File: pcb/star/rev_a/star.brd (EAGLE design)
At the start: 47 x 40 mm, 42 parts, among them J2 TC2030-JLINK-NL, J3 MICRO_USB_B_HIROSE_ZX62-B-5PA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, J4 TC2030-JLINK-NL, U2 LTC4065, U3 TRIPOINT, U4 TPS715AXX, U5 NRF51822QF, X1 EPSON-FA-128

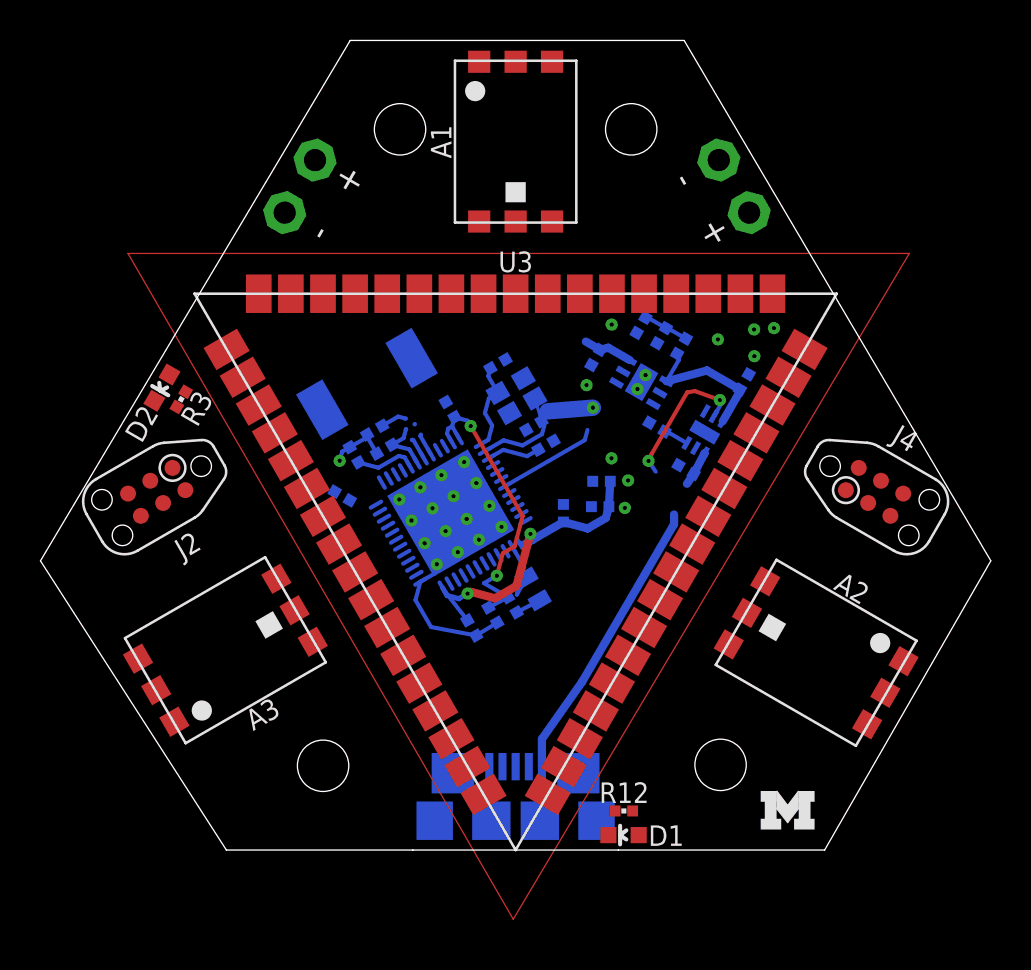
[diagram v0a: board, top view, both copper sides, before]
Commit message: fixed up dimensions
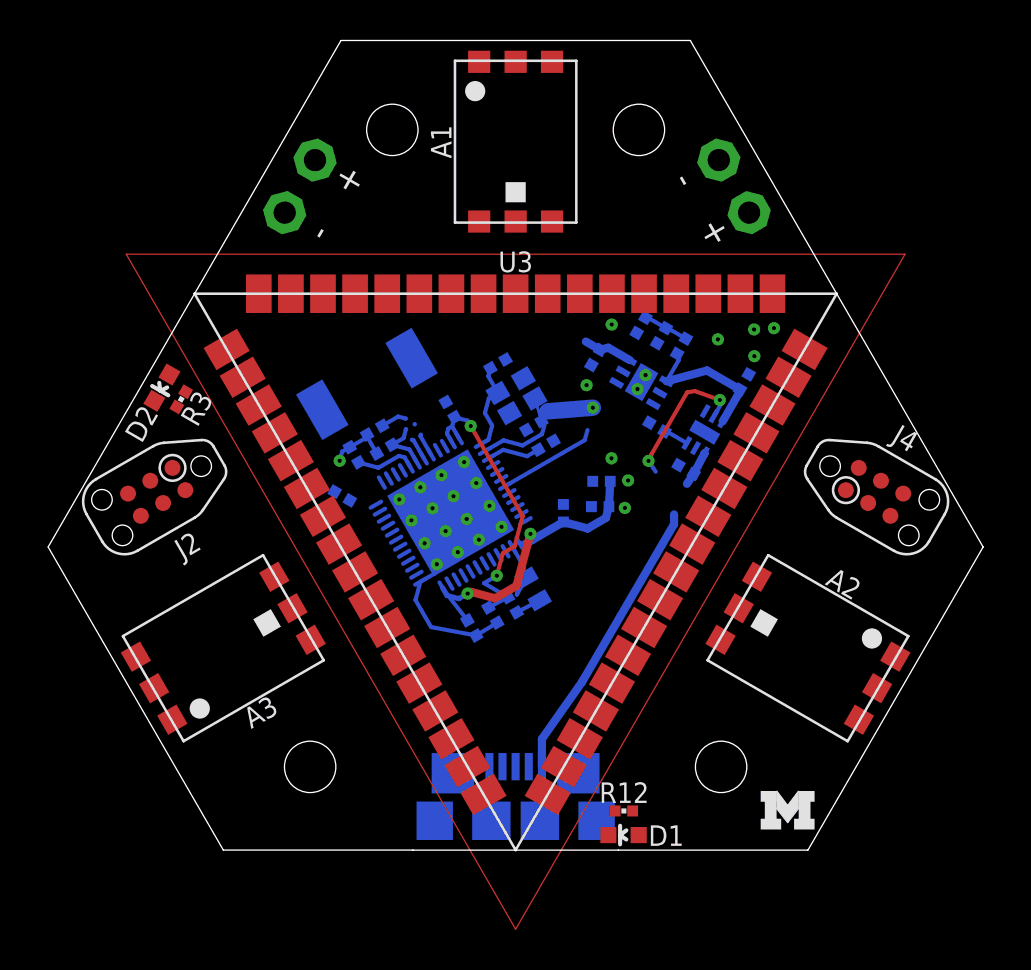
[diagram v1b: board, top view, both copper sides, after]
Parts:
- moved A2 0.47 mm to (14.5, -8.36)
- moved A3 0.14 mm to (-14.5, -8.36)
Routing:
- net GND: track 127.5 -> 128.1 mm
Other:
- board size 47 x 40 mm -> 46.2 x 40 mm
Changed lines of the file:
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@@
 <board>
 <plain>
-<wire x1="-8.178803125" y1="21.693628125" x2="8.331196875" y2="21.693628125" width="0" layer="20"/>
-<wire x1="8.331196875" y1="21.693628125" x2="23.494996875" y2="-4.03656875" width="0" layer="20"/>
-<wire x1="23.494996875" y1="-4.03656875" x2="15.27718125" y2="-18.33676875" width="0" layer="20"/>
-<wire x1="-14.301196875" y1="-18.33676875" x2="-23.495003125" y2="-4.036575" width="0" layer="20"/>
-<wire x1="-23.495003125" y1="-4.036575" x2="-8.178803125" y2="21.693628125" width="0" layer="20"/>
-<wire x1="-14.301196875" y1="-18.33676875" x2="-5.080003125" y2="-18.33676875" width="0" layer="20"/>
-<wire x1="5.08" y1="-18.33676875" x2="15.27718125" y2="-18.33676875" width="0" layer="20"/>
-<hole x="10.13289375" y="-14.124225" drill="2.54"/>
-<hole x="-9.52028125" y="-14.169271875" drill="2.54"/>
-<hole x="-5.715003125" y="17.299428125" drill="2.54"/>
-<hole x="5.714996875" y="17.29943125" drill="2.54"/>
+<wire x1="-8.636" y1="21.6916" x2="8.636" y2="21.6916" width="0" layer="20"/>
+<wire x1="8.636" y1="21.6916" x2="23.114" y2="-3.3528" width="0" layer="20"/>
+<wire x1="23.114" y1="-3.3528" x2="14.4526" y2="-18.3388" width="0" layer="20"/>
+<wire x1="-14.4526" y1="-18.33676875" x2="-23.114" y2="-3.3528" width="0" layer="20"/>
+<wire x1="-23.114" y1="-3.3528" x2="-8.636" y2="21.6916" width="0" layer="20"/>
+<wire x1="-14.4526" y1="-18.33676875" x2="-5.08" y2="-18.33676875" width="0" layer="20"/>
+<wire x1="5.08" y1="-18.3388" x2="14.4526" y2="-18.3388" width="0" layer="20"/>
+<hole x="10.16" y="-14.224" drill="2.54"/>
+<hole x="-10.16" y="-14.224" drill="2.54"/>
+<hole x="-6.096" y="17.272" drill="2.54"/>
+<hole x="6.096" y="17.272" drill="2.54"/>
 </plain>
 <attributes>
@@
 </autorouter>
 <elements>
-<element name="A1" library="chips" package="TAIYO-YUDEN-AH086M" value="TAIYO-YUDEN-AH086M" x="0" y="16.68983125" smashed="yes">
-<attribute name="DIGIKEY" value="587-2204-1-ND" x="16.509996875" y="11.609828125" size="1.778" layer="27" display="off"/>
-<attribute name="NAME" x="-3.17323125" y="16.6878" size="1.016" layer="25" font="vector" ratio="12" rot="R90" align="bottom-center"/>
-</element>
-<element name="A2" library="chips" package="TAIYO-YUDEN-AH086M" value="TAIYO-YUDEN-AH086M" x="14.858996875" y="-8.58316875" smashed="yes" rot="R240">
-<attribute name="DIGIKEY" value="587-2204-1-ND" x="-0.970409375" y="-25.840509375" size="1.778" layer="27" rot="R240" display="off"/>
-<attribute name="NAME" x="16.39176875" y="-5.829878125" size="1.016" layer="25" font="vector" ratio="12" rot="R330" align="bottom-center"/>
-</element>
-<element name="A3" library="chips" package="TAIYO-YUDEN-AH086M" value="TAIYO-YUDEN-AH086M" x="-14.351003125" y="-8.45616875" smashed="yes" rot="R120">
-<attribute name="DIGIKEY" value="587-2204-1-ND" x="-8.307925" y="14.09690625" size="1.778" layer="27" rot="R120" display="off"/>
-<attribute name="NAME" x="-12.767434375" y="-11.162728125" size="1.016" layer="25" font="vector" ratio="12" rot="R210" align="bottom-center"/>
+<element name="A1" library="chips" package="TAIYO-YUDEN-AH086M" value="TAIYO-YUDEN-AH086M" x="0" y="16.6878" smashed="yes">
+<attribute name="DIGIKEY" value="587-2204-1-ND" x="16.509996875" y="11.607796875" size="1.778" layer="27" display="off"/>
+<attribute name="NAME" x="-3.17323125" y="16.68576875" size="1.016" layer="25" font="vector" ratio="12" rot="R90" align="bottom-center"/>
+</element>
+<element name="A2" library="chips" package="TAIYO-YUDEN-AH086M" value="TAIYO-YUDEN-AH086M" x="14.4526" y="-8.3566" smashed="yes" rot="R240">
+<attribute name="DIGIKEY" value="587-2204-1-ND" x="-1.37680625" y="-25.613940625" size="1.778" layer="27" rot="R240" display="off"/>
+<attribute name="NAME" x="15.985371875" y="-5.603309375" size="1.016" layer="25" font="vector" ratio="12" rot="R330" align="bottom-center"/>
+</element>
+<element name="A3" library="chips" package="TAIYO-YUDEN-AH086M" value="TAIYO-YUDEN-AH086M" x="-14.4526" y="-8.3566" smashed="yes" rot="R120">
+<attribute name="DIGIKEY" value="587-2204-1-ND" x="-8.409521875" y="14.196475" size="1.778" layer="27" rot="R120" display="off"/>
+<attribute name="NAME" x="-12.86903125" y="-11.063159375" size="1.016" layer="25" font="vector" ratio="12" rot="R210" align="bottom-center"/>
 </element>
 <element name="X1" library="crystals" package="FA-128" value="EPSON-FA-128" x="0.040640625" y="4.12666875" smashed="yes" rot="MR150">
@@
 <attribute name="VALUE" x="-17.914746875" y="5.944984375" size="0.4064" layer="27" rot="R240"/>
 </element>
-<element name="J3" library="connector" package="USB_MICRO_B-HIROSE-ZX62-B-5PA(11)" value="MICRO_USB_B_HIROSE_ZX62-B-5PA(11)" x="0" y="-18.33676875" rot="MR0">
-<attribute name="MOUSER" value="798-ZX62-B-5PA11" x="0" y="-18.33676875" size="1.778" layer="28" rot="MR0" display="off"/>
-<attribute name="NEWARK" value="86P8793" x="0" y="-18.33676875" size="1.778" layer="28" rot="MR0" display="off"/>
-<attribute name="DIGIKEY" value="H11634CT-ND" x="0" y="-18.33676875" size="1.778" layer="28" rot="MR0" display="off"/>
+<element name="J3" library="connector" package="USB_MICRO_B-HIROSE-ZX62-B-5PA(11)" value="MICRO_USB_B_HIROSE_ZX62-B-5PA(11)" x="0" y="-18.3388" rot="MR0">
+<attribute name="MOUSER" value="798-ZX62-B-5PA11" x="0" y="-18.3388" size="1.778" layer="28" rot="MR0" display="off"/>
+<attribute name="NEWARK" value="86P8793" x="0" y="-18.3388" size="1.778" layer="28" rot="MR0" display="off"/>
+<attribute name="DIGIKEY" value="H11634CT-ND" x="0" y="-18.3388" size="1.778" layer="28" rot="MR0" display="off"/>
 </element>
 <element name="U3" library="tripoint" package="TRIPOINT" value="TRIPOINT" x="0" y="0"/>
@@
 <wire x1="3.819071875" y1="3.535628125" x2="1.5793875" y2="3.35624375" width="0.8128" layer="16"/>
 <contactref element="J3" pad="5"/>
-<wire x1="-19.167390625" y1="11.162290625" x2="-0.117390625" y2="-21.756109375" width="0" layer="1"/>
-<wire x1="-0.117390625" y1="-21.756109375" x2="19.466009375" y2="11.162290625" width="0" layer="1"/>
-<wire x1="19.466009375" y1="11.162290625" x2="-19.167390625" y2="11.162290625" width="0" layer="1"/>
+<wire x1="-19.2532" y1="11.1252" x2="0" y2="-22.2504" width="0" layer="1"/>
+<wire x1="0" y1="-22.2504" x2="19.2532" y2="11.1252" width="0" layer="1"/>
+<wire x1="19.2532" y1="11.1252" x2="-19.2532" y2="11.1252" width="0" layer="1"/>
 <contactref element="U$4" pad="N"/>
 <contactref element="U$3" pad="N"/>
@@
 <wire x1="-6.862209375" y1="1.268534375" x2="-4.9900625" y2="2.718665625" width="0" layer="19" extent="16-16"/>
 <wire x1="-8.19645625" y1="-1.045490625" x2="-8.70006875" y2="0.911309375" width="0" layer="19" extent="16-16"/>
-<wire x1="-1.3" y1="-14.21176875" x2="-1.952625" y2="-7.729175" width="0" layer="19" extent="16-16"/>
-<wire x1="19.466009375" y1="11.162290625" x2="12.7727375" y2="7.466778125" width="0" layer="19" extent="1-1"/>
-<wire x1="-11.418" y1="13.178959375" x2="-19.167390625" y2="11.162290625" width="0" layer="19" extent="1-1"/>
+<wire x1="-1.3" y1="-14.2138" x2="-1.952625" y2="-7.729175" width="0" layer="19" extent="16-16"/>
+<wire x1="19.2532" y1="11.1252" x2="12.7727375" y2="7.466778125" width="0" layer="19" extent="1-1"/>
+<wire x1="-11.418" y1="13.178959375" x2="-19.2532" y2="11.1252" width="0" layer="19" extent="1-1"/>
 <wire x1="18.52935625" y1="-1.811671875" x2="11.525375" y2="5.18295625" width="0" layer="19" extent="1-16"/>
 <wire x1="-19.16435625" y1="-0.71181875" x2="-8.70006875" y2="0.911309375" width="0" layer="19" extent="1-1"/>
@@
 <wire x1="8.80435" y1="0.26226875" x2="8.4719375" y2="-0.227078125" width="0.4064" layer="16"/>
 <contactref element="J3" pad="1"/>
-<wire x1="1.3" y1="-14.21176875" x2="1.3" y2="-12.84571875" width="0.4064" layer="16"/>
+<wire x1="1.3" y1="-14.2138" x2="1.3" y2="-12.84571875" width="0.4064" layer="16"/>
 <wire x1="1.3" y1="-12.84571875" x2="3.286209375" y2="-10.021309375" width="0.4064" layer="16"/>
 <wire x1="3.286209375" y1="-10.021309375" x2="7.832809375" y2="-2.223509375" width="0.4064" layer="16"/>
 <wire x1="7.832809375" y1="-2.223509375" x2="7.832809375" y2="-1.743046875" width="0.4064" layer="16"/>
-<wire x1="1.3" y1="-14.21176875" x2="4.918759375" y2="-16.402353125" width="0" layer="19" extent="1-16"/>
+<wire x1="1.3" y1="-14.2138" x2="4.918759375" y2="-16.402353125" width="0" layer="19" extent="1-16"/>
 <wire x1="8.4719375" y1="-0.227078125" x2="7.832809375" y2="-1.743046875" width="0" layer="19" extent="16-16"/>
 </signal>

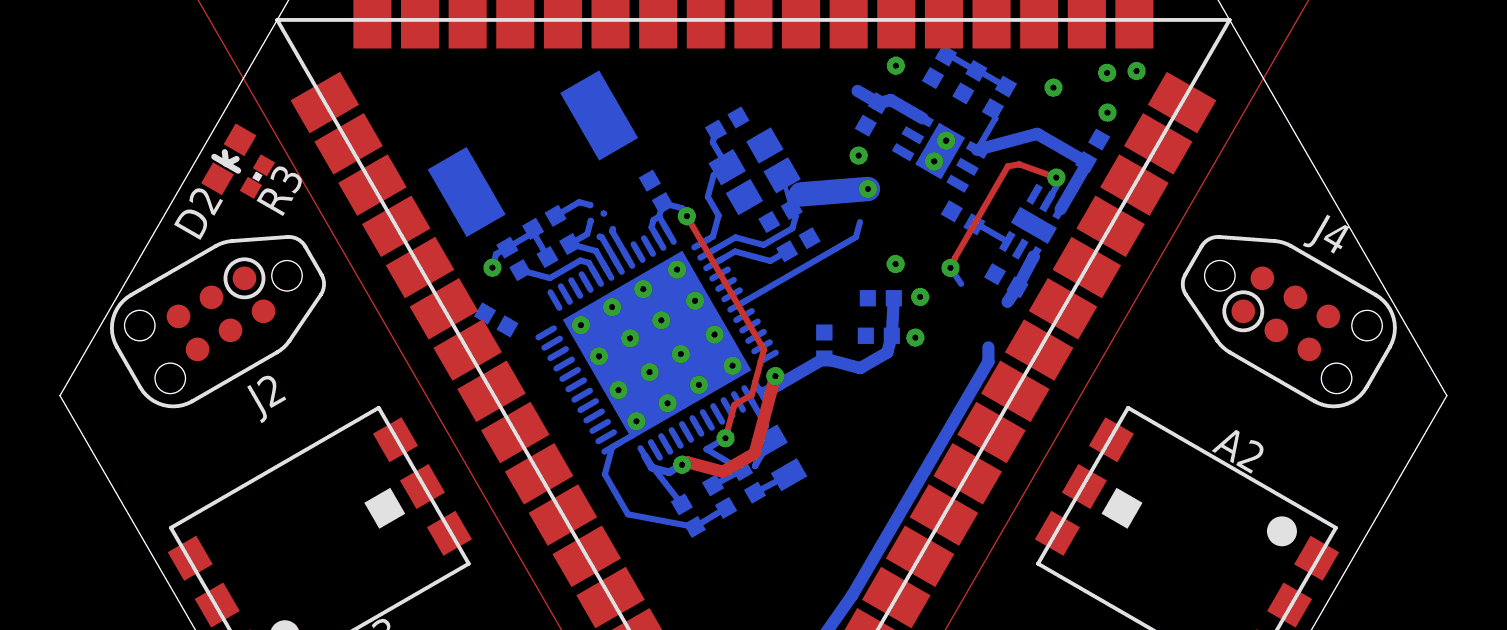
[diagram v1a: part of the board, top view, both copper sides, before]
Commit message: much farther on anchor
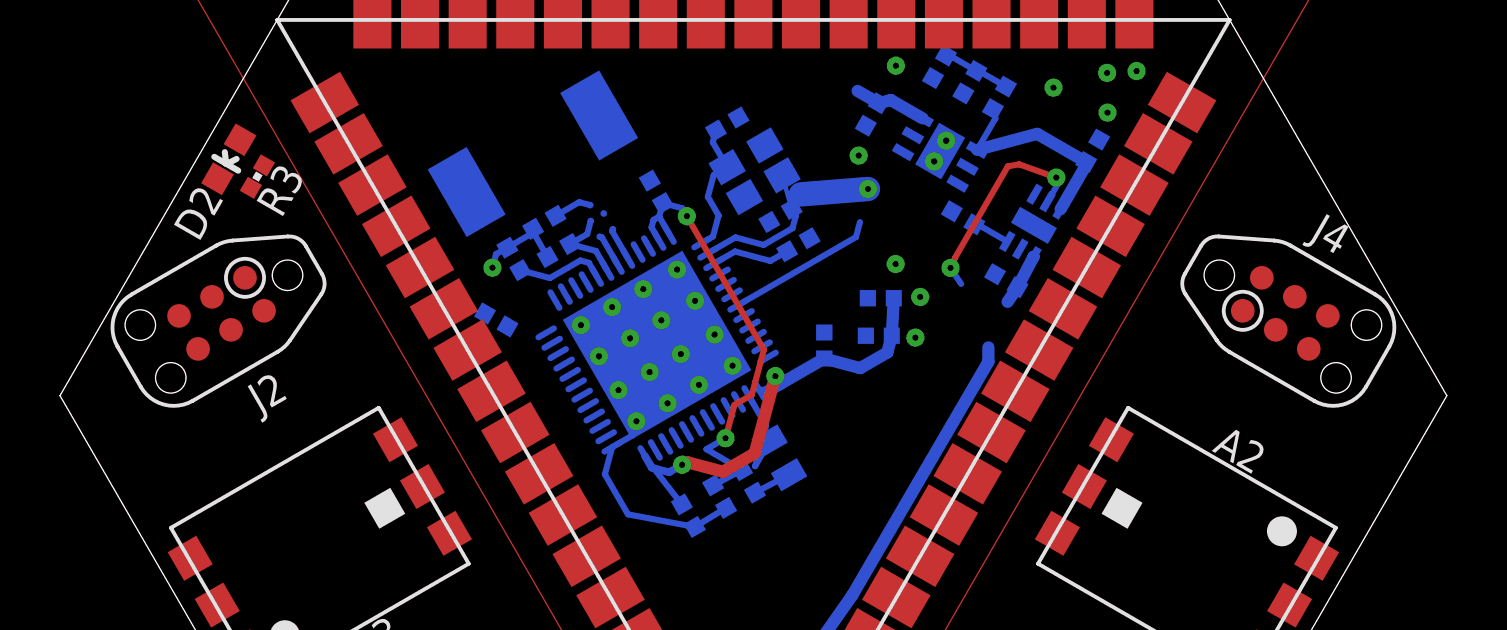
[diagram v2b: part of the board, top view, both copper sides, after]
